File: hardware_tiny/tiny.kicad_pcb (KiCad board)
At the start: 2 copper layers, 45 x 23 mm, 35 parts, among them P1 USB_OTG, P2 CONN_02X05, P3 CONN_01X05, P4 CONN_01X05, U1 AMS1117-3.3, U2 STM32F103CB, Y1 8M

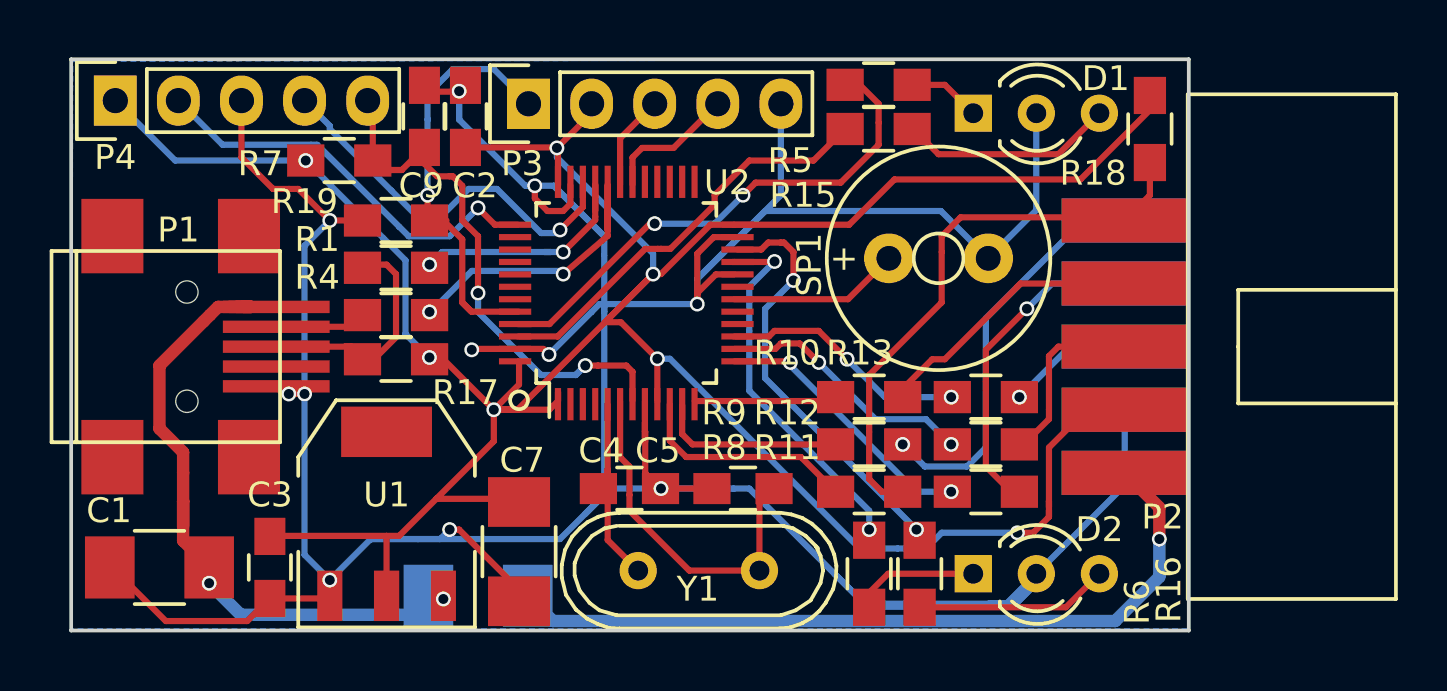
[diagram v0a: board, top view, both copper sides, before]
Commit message: edit
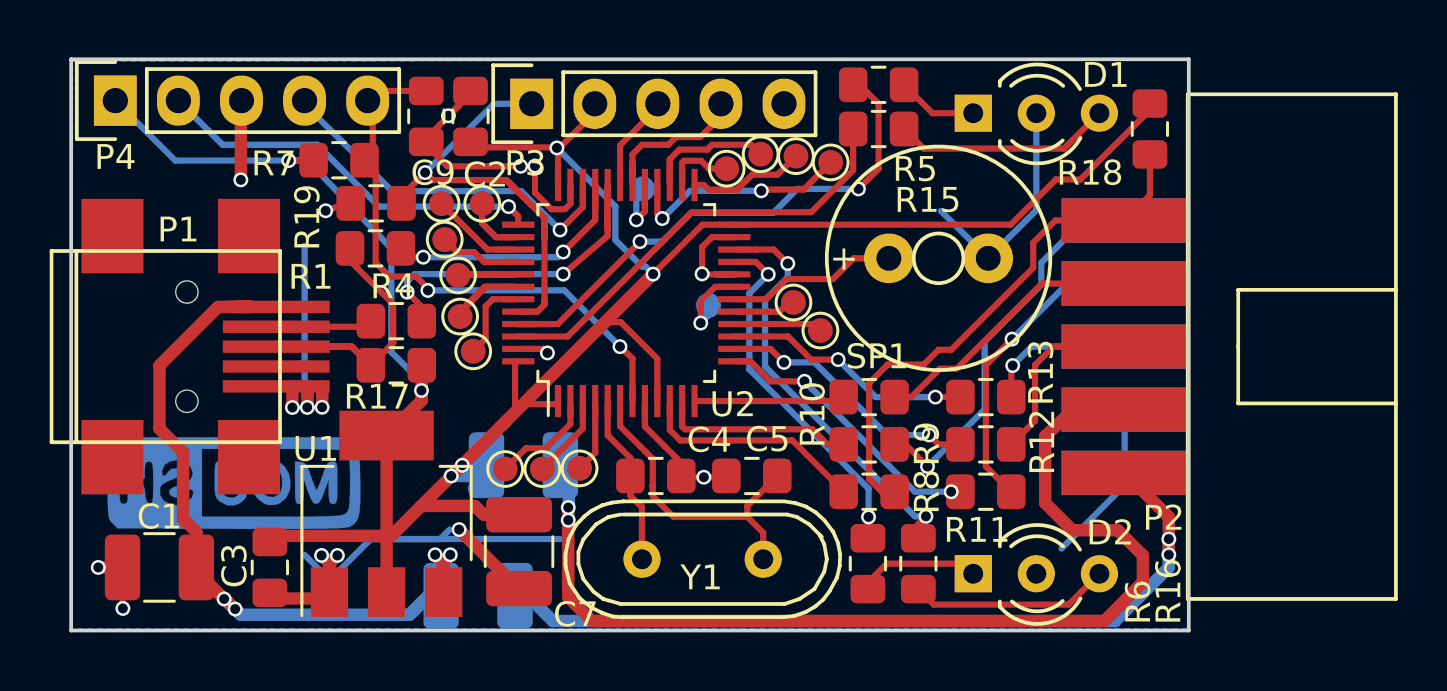
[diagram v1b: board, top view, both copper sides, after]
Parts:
- removed LOGO: LOGO, footprints:mcush_logo
- added F2: 200mA, Resistor_SMD:R_1210_3225Metric_Pad1.42x2.65mm_HandSolder, B.Cu at (108.4, 117.8)
- added LOGO1: MCUSH, logo:mcush_txt_logo, B.Cu at (96.7, 118.5)
- added TP1: D6, TestPoint:TestPoint_Pad_D1.0mm, F.Cu at (120.3, 112.4)
- added TP10: D8, TestPoint:TestPoint_Pad_D1.0mm, B.Cu at (113.2, 106.7)
- added TP11: PA15, TestPoint:TestPoint_Pad_D1.0mm, F.Cu at (106.7, 107.3)
- added TP12: PB1, TestPoint:TestPoint_Pad_D1.0mm, B.Cu at (115.8, 111.4)
- added TP13: PB3, TestPoint:TestPoint_Pad_D1.0mm, F.Cu at (105.1, 107.3)
- added TP14: PB4, TestPoint:TestPoint_Pad_D1.0mm, F.Cu at (105.2, 108.7)
- added TP15: PB5, TestPoint:TestPoint_Pad_D1.0mm, F.Cu at (105.8, 110.2)
- added TP16: PB6, TestPoint:TestPoint_Pad_D1.0mm, F.Cu at (105.8, 111.8)
- added TP17: PB7, TestPoint:TestPoint_Pad_D1.0mm, F.Cu at (106.4, 113.2)
- added TP2: D7, TestPoint:TestPoint_Pad_D1.0mm, F.Cu at (119.3, 111.3)
- added TP3: C13, TestPoint:TestPoint_Pad_D1.0mm, F.Cu at (107.6, 118.0)
- added TP4: C14, TestPoint:TestPoint_Pad_D1.0mm, F.Cu at (109.1, 118.0)
- added TP5: C15, TestPoint:TestPoint_Pad_D1.0mm, F.Cu at (110.6, 117.9)
- added TP6: CS, TestPoint:TestPoint_Pad_D1.0mm, F.Cu at (119.4, 105.4)
- added TP7: SCK, TestPoint:TestPoint_Pad_D1.0mm, F.Cu at (116.6, 105.9)
- added TP8: MISO, TestPoint:TestPoint_Pad_D1.0mm, F.Cu at (117.9, 105.3)
- added TP9: MOSI, TestPoint:TestPoint_Pad_D1.0mm, F.Cu at (120.8, 105.6)
- C1, C7: footprint Capacitors_SMD:C_1210_HandSoldering -> Capacitor_SMD:C_1210_3225Metric_Pad1.42x2.65mm_HandSolder
- C2, C3, C4, C5, C9: footprint Capacitors_SMD:C_0805_HandSoldering -> Capacitor_SMD:C_0805_2012Metric_Pad1.15x1.40mm_HandSolder
- F1: footprint Resistors_SMD:R_1210_HandSoldering -> Resistor_SMD:R_1210_3225Metric_Pad1.42x2.65mm_HandSolder
- R1, R10, R11, R12, R13, R15, R16, R17, R18, R19, R4, R5, R6, R7, R8, R9: footprint Resistors_SMD:R_0805_HandSoldering -> Resistor_SMD:R_0805_2012Metric_Pad1.15x1.40mm_HandSolder
- U1: footprint footprints:SOT-223 -> Package_TO_SOT_SMD:SOT-223-3_TabPin2
- U2: footprint footprints:LQFP-48_7x7mm_Pitch0.5mm_HandSoldering -> Package_QFP:LQFP-48_7x7mm_P0.5mm
- moved C4 1.18 mm to (113.7, 118.2)
- moved R1 1.14 mm to (102.4, 109.1)
- moved R19 1.06 mm to (102.4, 107.3)
- moved C5 0.62 mm to (117.6, 118.2)
- moved Y1 0.48 mm to (115.6, 121.6)
- moved R16 0.41 mm to (124.3, 121.8)
- moved R6 0.41 mm to (122.3, 121.8)
- moved R17 0.24 mm to (103.3, 113.8)
- moved R4 0.24 mm to (103.3, 112.0)
- moved C2 0.20 mm to (106.2, 103.8)
- moved P3 0.13 mm to (108.7, 103.3)
- moved C9 0.08 mm to (104.5, 103.8), turned to 90 degrees
- turned U1 to 90 degrees
- turned U2 to 90 degrees
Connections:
- P2 pad 7: +3V3 -> /3.3V_OUT
- U2 pad 16: Net-(U2-Pad16) -> /D6
- U2 pad 17: Net-(U2-Pad17) -> /D7
- U2 pad 19: Net-(U2-Pad19) -> /PB1
- U2 pad 2: Net-(U2-Pad2) -> /C13
- U2 pad 29: Net-(U2-Pad29) -> /D8
- U2 pad 3: Net-(U2-Pad3) -> /C14
- U2 pad 38: Net-(U2-Pad38) -> /PA15
- U2 pad 39: Net-(U2-Pad39) -> /PB3
- U2 pad 4: Net-(U2-Pad4) -> /C15
- U2 pad 40: Net-(U2-Pad40) -> /PB4
- U2 pad 41: Net-(U2-Pad41) -> /PB5
- U2 pad 42: Net-(U2-Pad42) -> /PB6
- U2 pad 43: Net-(U2-Pad43) -> /PB7
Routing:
- net GND: track 182.9 -> 85.6 mm, vias 11 -> 16
- net /3.3V_OUT: track 0.00 -> 42.6 mm, vias 0 -> 2
- net +3V3: track 130.0 -> 109.2 mm, vias 7 -> 6
- net /SPI_MOSI: track 0.00 -> 9.14 mm, vias 0 -> 2
- net +5V: track 27.4 -> 34.5 mm, vias 2 -> 4
- net /PB5: track 0.00 -> 6.47 mm
- net /SPI_MISO: track 0.00 -> 5.96 mm
- net /D8: track 0.00 -> 5.67 mm, vias 0 -> 1
- net /PB6: track 0.00 -> 5.34 mm
- net /SPI_CS: track 0.00 -> 5.05 mm
- net /USB_DP: track 10.5 -> 15.2 mm
- net /PA15: track 0.00 -> 4.23 mm
- net /C13: track 0.00 -> 4.17 mm
- net /PB3: track 0.00 -> 3.73 mm
- net /D6: track 0.00 -> 3.65 mm
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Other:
- net class 5V_PWR removed
- net class PWR added: clearance 0.2, trace_width 0.5, via_dia 0.6, via_drill 0.4
- board text added: "For more infomation, visit:"
- board text added: "https://github.com/pengshulin/mcush"
